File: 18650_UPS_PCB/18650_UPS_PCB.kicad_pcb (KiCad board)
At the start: 4 copper layers, 90 x 22 mm, 54 parts, among them J1 USB_B_Micro, J2 Conn_02x04_Odd_Even, J3 USB_A, SW1 SW_SPDT, SW2 ALPSALPINE_SKRHADE011, SW3 SW_SPDT, SW4 SW_SPDT, SW5 SW_SPDT, U1 STLINK-V3MINI, U10 LR9102G-xx, U2 R5478, U3 STC4054, U4 FS8205A, U5 ME2188Cxx, U6 XC9236Axx, U7 INA219AxD, U8 SSD1306_128_32, U9 STM32F030F4Px

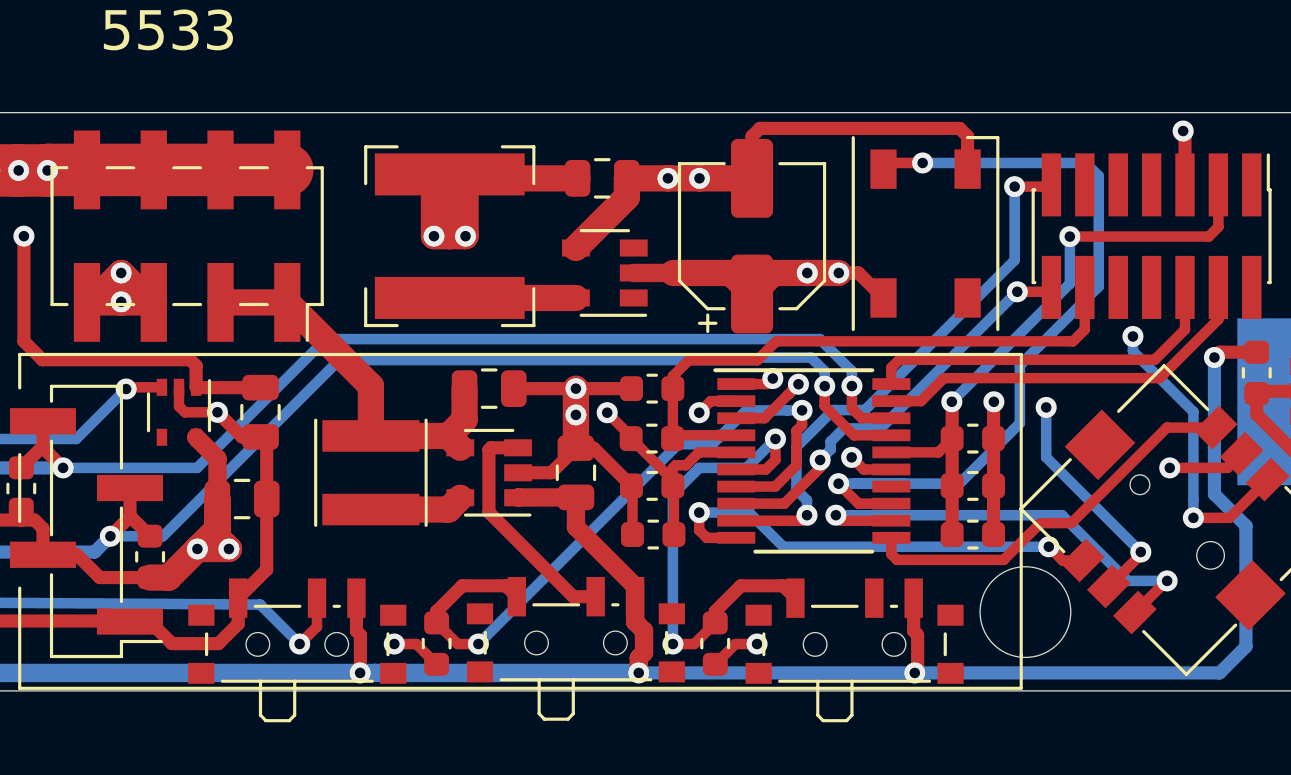
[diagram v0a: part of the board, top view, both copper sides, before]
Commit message: routing done
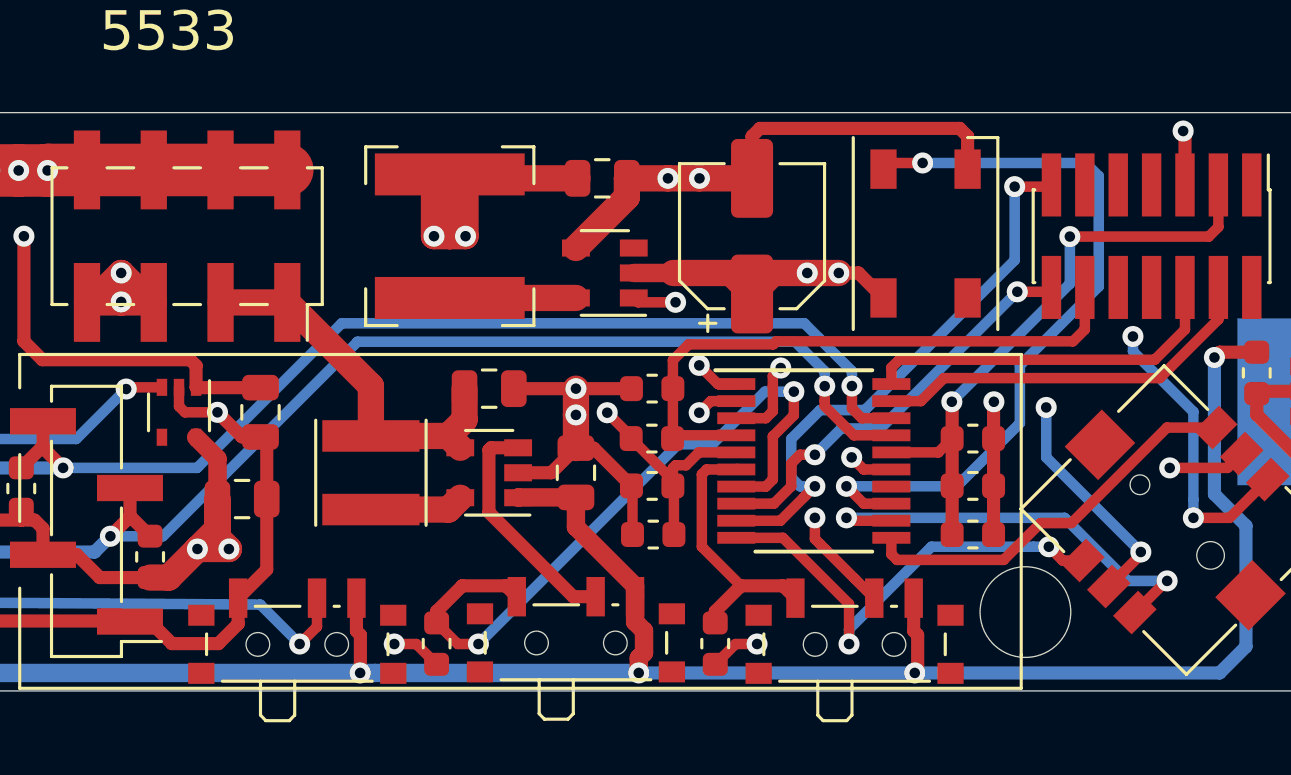
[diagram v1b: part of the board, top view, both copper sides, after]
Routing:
- net BoostCE: track 0.00 -> 17.2 mm, vias 0 -> 2
- net PA0: track 19.0 -> 10.4 mm, vias 2 -> 0
- net PA7: track 31.2 -> 28.7 mm
- net PA6: track 17.6 -> 16.7 mm
- net USART1_RX: track 21.0 -> 21.6 mm
- net I2C1_SDA: track 51.4 -> 51.9 mm
